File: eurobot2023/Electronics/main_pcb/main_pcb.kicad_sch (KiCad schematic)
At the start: 55 parts, among them IC1 CD74HCT125M96, IC2 SN74LVC126ADR, J1 PI40HAT, J10 Conn_01x02_Male, J11 MagneticEncoder, J12 Conn_01x07_Male, J13 MagneticEncoder, J14 Conn_01x03_Male, J15 Conn_01x02_Male, J16 Conn_02x02_Odd_Even, J17 Conn_02x02_Odd_Even, J18 Conn_02x02_Odd_Even, J2 Conn_01x02_Male, J20 Conn_01x03_Male, J21 Conn_01x03_Male, J24 Conn_01x03_Male, J3 Conn_01x02_Male, J4 Conn_01x02_Male, J5 Conn_01x02_Male, J6 Conn_01x02_Male, J7 Conn_01x02_Male, J8 Conn_01x02_Male, J9 22-03-5035, P1 R-78Bxx-2.0, P2 Amazon 10A stepdown, Q1 2SK4017_Q_, Q2 2SK4017_Q_, Q3 2SK4017_Q_, Q4 2SK4017_Q_, Q5 2SK4017_Q_, Q6 2SK4017_Q_, U1 MCP2515-xSO, U2 TJA1049T, U3 PCA9306D, U4 Pololu_MAX14870, U5 PCA9685PW, U6 Pololu_MAX14870

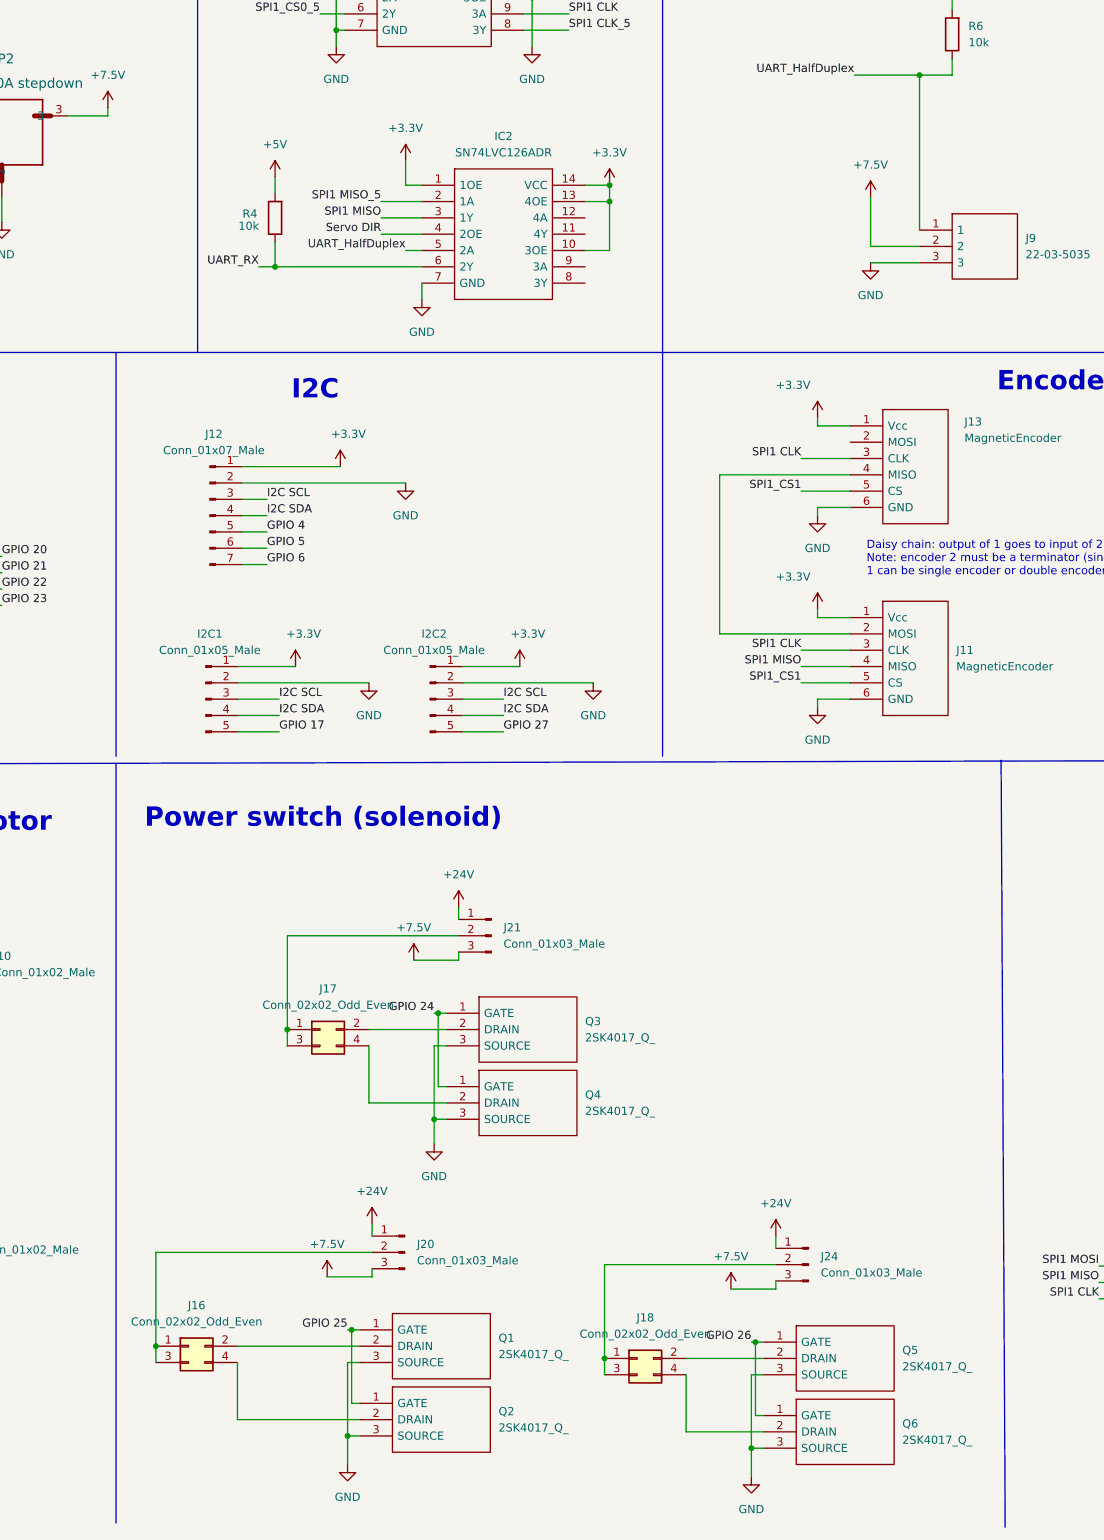
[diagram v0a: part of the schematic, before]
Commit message: Fix main pcb
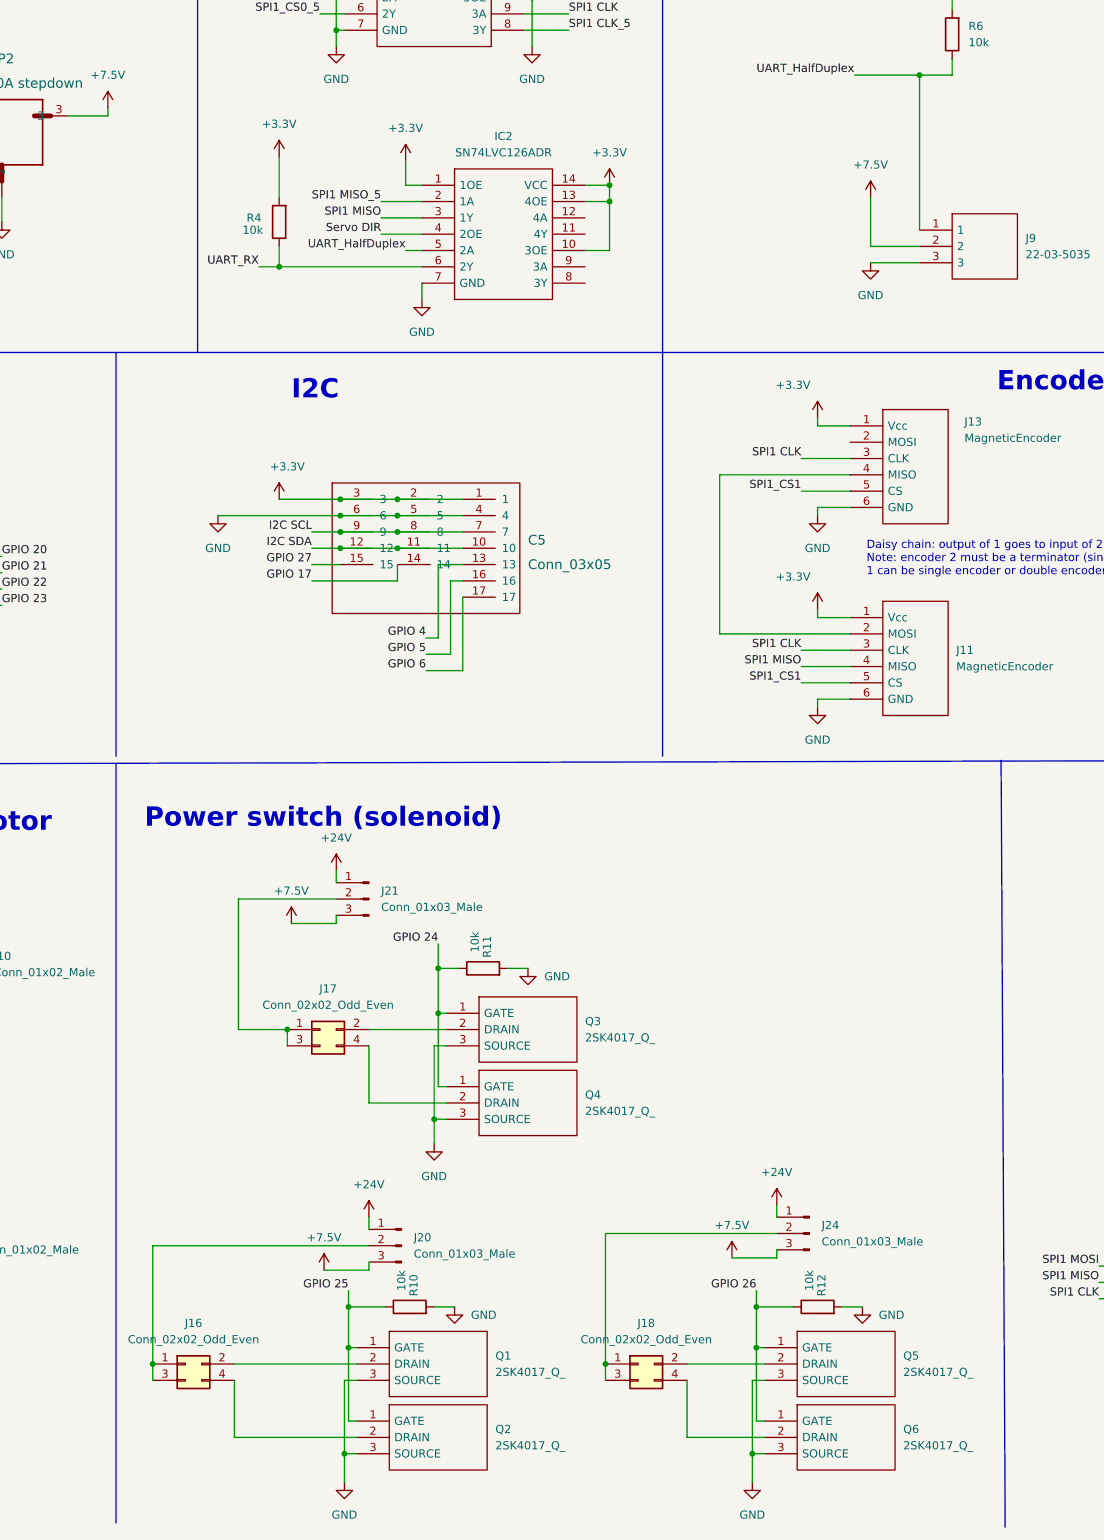
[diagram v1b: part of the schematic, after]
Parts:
- removed I2C1, I2C2: Conn_01x05_Male, Connector_PinHeader_2.54mm:PinHeader_1x05_P2.54mm_Vertical, symbol Connector:Conn_01x05_Male
- removed J12: Conn_01x07_Male, Connector_PinHeader_2.54mm:PinHeader_1x07_P2.54mm_Vertical, symbol Connector:Conn_01x07_Male
- added C5: Conn_03x05, MiAM:Pin_Header_Straight_3x05_Pitch2.54mm, symbol MiAM:Conn_03x05
- added R10, R11, R12: 10k, Resistor_SMD:R_0805_2012Metric, symbol Device:R
- IC2: RS Part Number 662-8601 -> SN74LVC126ADR
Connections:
- net +3.3V: now also R4.2, C5.1, C5.2, C5.3
- net +5V: no longer R4.2
- net GND: now also C5.4, C5.5, C5.6, R10.2, R11.2, R12.2
- net GPIO 17: now also C5.14
- net GPIO 24: now also R11.1
- net GPIO 25: now also R10.1
- net GPIO 26: now also R12.1
- net GPIO 27: now also C5.15
- net GPIO 4: now also C5.13
- net GPIO 5: now also C5.16
- net GPIO 6: now also C5.17
- net I2C SCL: now also C5.7, C5.8, C5.9
- net I2C SDA: now also C5.10, C5.11, C5.12
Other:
- moved on the sheet: J16, J18, J20, J21, J24, Q1, Q2, Q5, Q6, R4
